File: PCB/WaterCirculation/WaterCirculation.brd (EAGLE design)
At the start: 67 x 52.1 mm, 27 parts, among them K1 G5V1, K2 G5V1, K3 G5V1, Q1 MPSA42, Q3 MPSA42

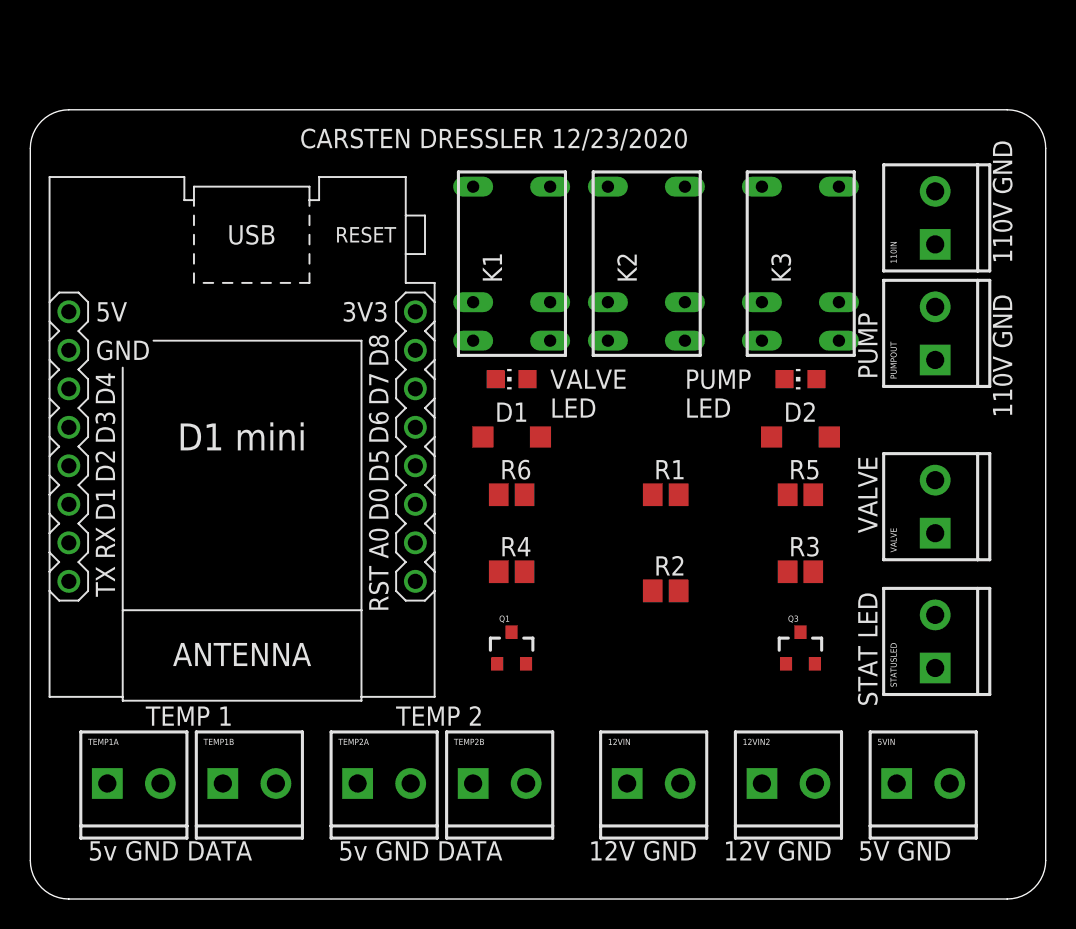
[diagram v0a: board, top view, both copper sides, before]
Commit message: final layout
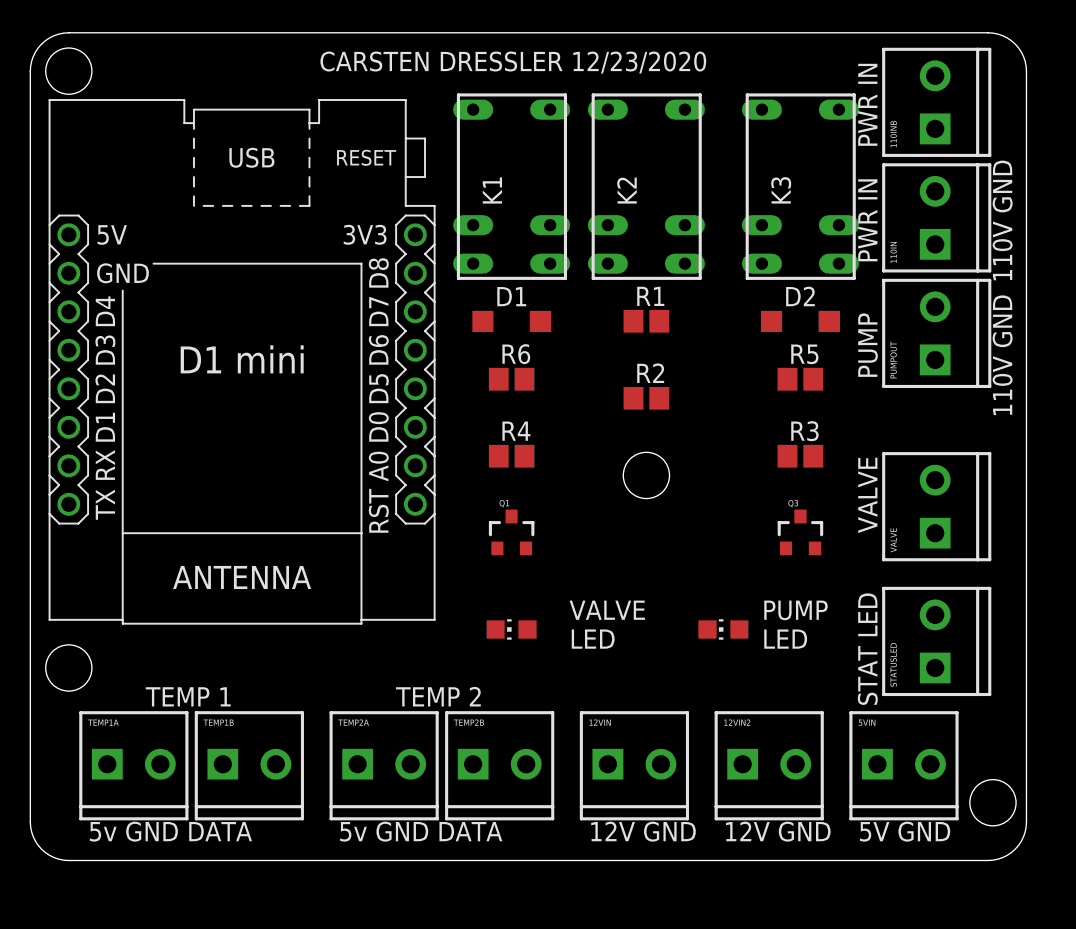
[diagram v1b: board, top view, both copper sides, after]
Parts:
- added 110INB: (no value), SparkFun-Connectors:SCREWTERMINAL-3.5MM-2
- moved LED2 17.3 mm to (45.7, 45.7)
- moved LED1 16.5 mm to (31.8, 45.7)
- moved R2 12.8 mm to (40.6, 61.0)
- moved R1 11.5 mm to (40.6, 66.0)
- moved D1 7.62 mm to (31.8, 66.0)
- moved D2 7.62 mm to (50.8, 66.0)
- moved Q1 7.62 mm to (31.8, 52.1)
- moved Q3 7.62 mm to (50.8, 52.1)
- moved R3 7.62 mm to (50.8, 57.1)
- moved R4 7.62 mm to (31.8, 57.1)
- moved R5 7.62 mm to (50.8, 62.2)
- moved R6 7.62 mm to (31.8, 62.2)
- moved K1 5.08 mm to (31.8, 74.9)
- moved K2 5.08 mm to (40.6, 74.9)
- moved K3 5.08 mm to (50.8, 74.9)
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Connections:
- net N$10: now also 110INB.1
- net N$6: now also 110INB.2
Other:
- board size 67 x 52.1 mm -> 65.7 x 54.6 mm
- board text added: "PWR IN"
